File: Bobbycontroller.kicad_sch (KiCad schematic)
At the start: 37 parts, among them J1 Conn_01x01_Male, J10 Conn_01x01, J11 Conn_01x01, J12 Conn_01x01, J2 Conn_01x01_Male, J3 Conn_01x01_Male, J4 Conn_01x01_Male, J5 Conn_01x01_Male, J6 Conn_01x01_Male, J7 -BATT, J8 +BATT, J9 Conn_01x01

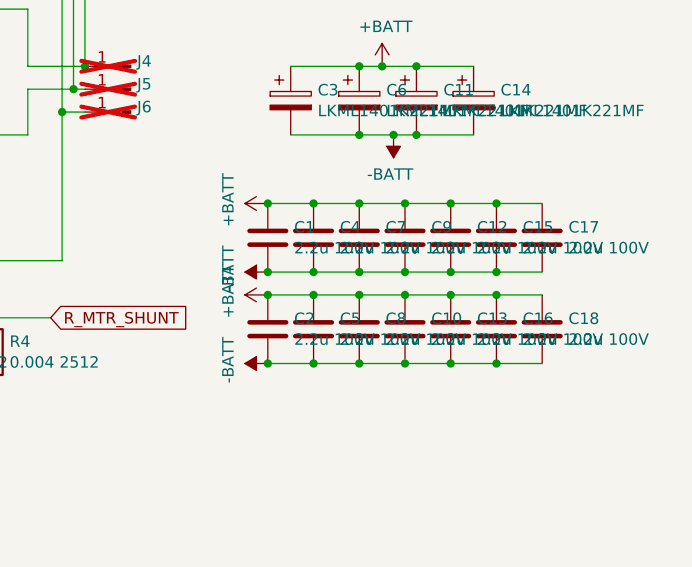
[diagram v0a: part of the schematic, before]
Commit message: update lcsc numbers
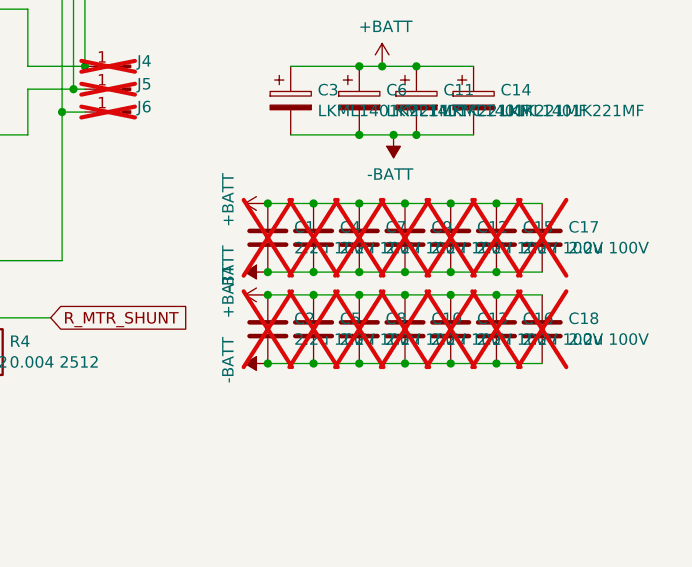
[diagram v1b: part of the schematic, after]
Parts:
- C1, C10, C12, C13, C15, C16, C17, C18, C2, C4, C5, C7, C8, C9: now not fitted; now left out of the parts list
- C11, C14, C3, C6: place hand -> (none)

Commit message: Exchanged more components, DNP and bridge 4.7R resistor, DNP 51V TVS diode
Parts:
- R1, R2, R3, R4: LCSC C270946 -> C46634448
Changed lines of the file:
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@@
 			)
 		)
-		(property "LCSC" "C270946"
+		(property "LCSC" "C46634448"
 			(at 215.9 67.31 0)
 			(effects
@@
 			)
 		)
-		(property "LCSC" "C270946"
+		(property "LCSC" "C46634448"
 			(at 205.74 67.31 0)
 			(effects
@@
 			)
 		)
-		(property "LCSC" "C270946"
+		(property "LCSC" "C46634448"
 			(at 215.9 157.48 0)
 			(effects
@@
 			)
 		)
-		(property "LCSC" "C270946"
+		(property "LCSC" "C46634448"
 			(at 205.74 157.48 0)
 			(effects
